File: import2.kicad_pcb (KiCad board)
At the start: 4 copper layers, 59.3 x 46.4 mm, 199 parts, among them P1 TP4057-42-SOT26-R, Q1 1, SW4 1.5m, U1 2, U14 62821, U15 1.8, U16 1, U2 ESP32-C6-MINI-1-N4

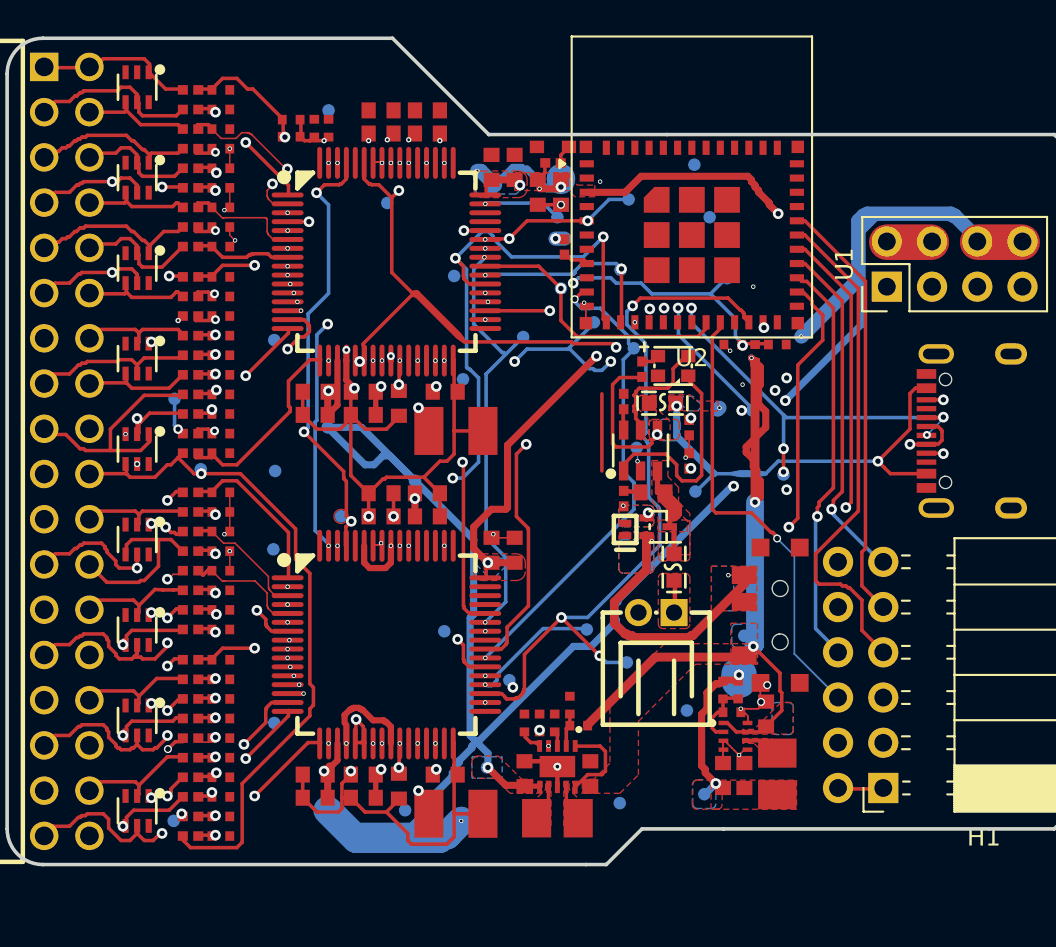
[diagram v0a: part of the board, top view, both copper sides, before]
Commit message: PCB update. DRC <300
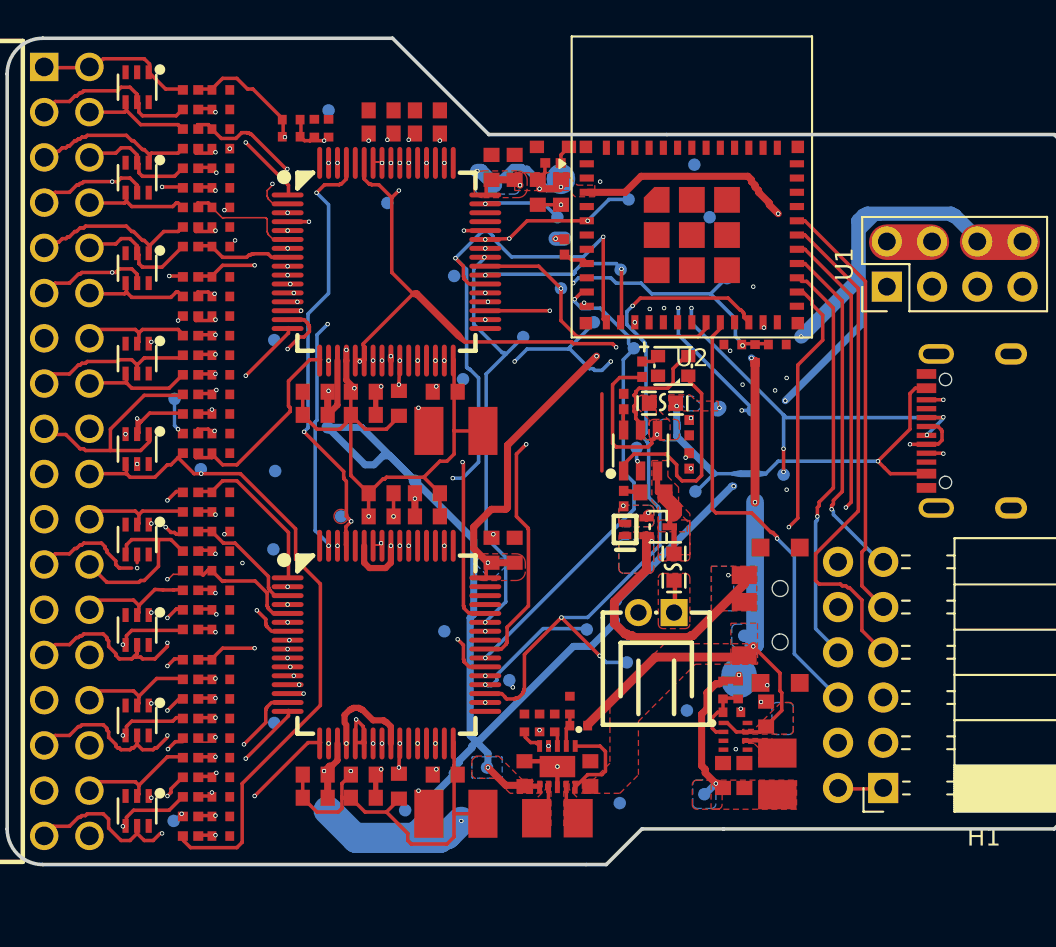
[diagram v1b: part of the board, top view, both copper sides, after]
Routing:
- net 3V3: track 155.7 -> 91.5 mm
- net GND: track 32.4 -> 13.6 mm
- net VIN: track 50.3 -> 40.9 mm
- net 5V: track 173.2 -> 166.9 mm
- added copper zone on F.Cu, net (none)
- added copper zone on F.Cu, net 3V3_ADC
- removed copper zone on F.Cu, net $1N290221
- removed copper zone on F.Cu, net $1N381046
- removed copper zone on F.Cu, net $1N381052
- removed copper zone on F.Cu, net $1N406824
